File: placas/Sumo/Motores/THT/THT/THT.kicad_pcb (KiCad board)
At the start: 2 copper layers, 69.7 x 54.7 mm, 3 parts, among them J1 Control Motores, J2 Conn_01x02_Male

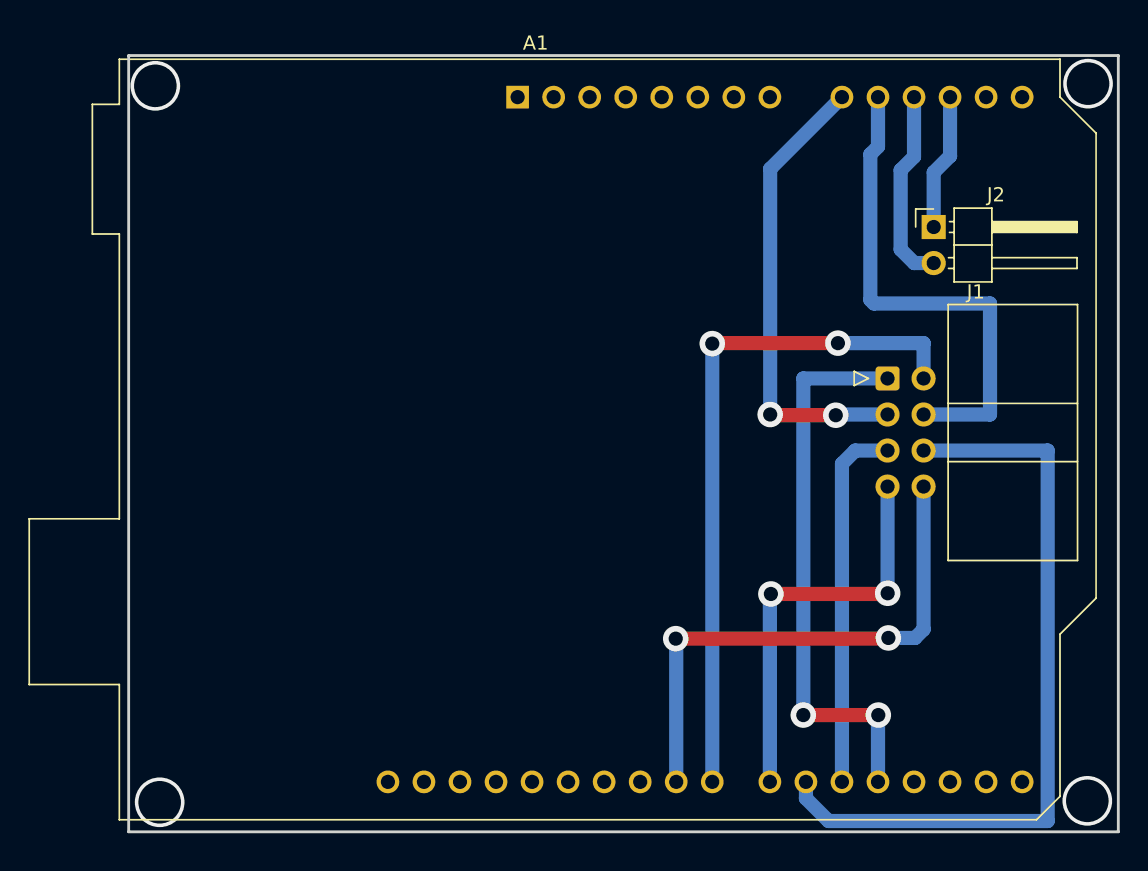
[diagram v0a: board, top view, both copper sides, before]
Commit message: CAMBIOS
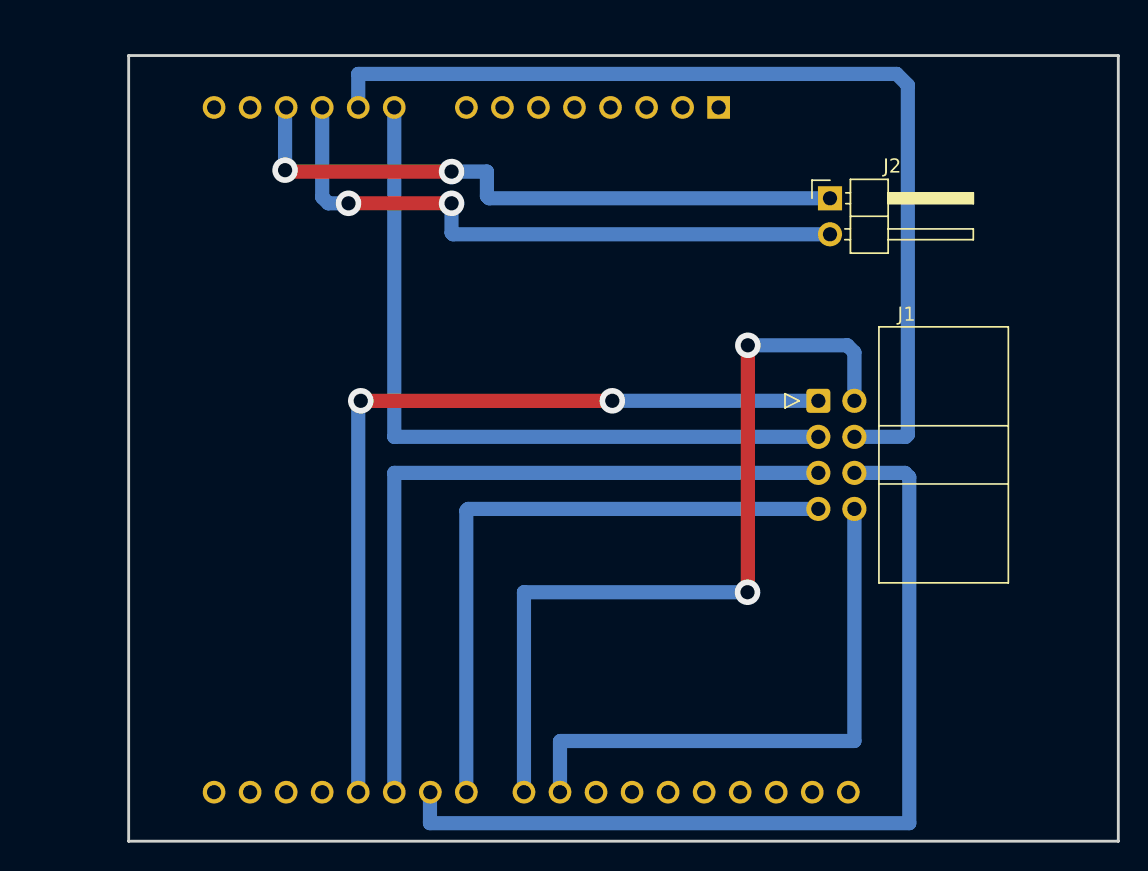
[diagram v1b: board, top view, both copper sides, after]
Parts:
- A1: moved to B.Cu
- moved A1 14.2 mm to (62.5, 20.2), turned to 180 degrees
- moved J2 7.58 mm to (70.4, 26.6)
- moved J1 5.12 mm to (69.5, 40.8)
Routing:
- net /C2: track 9.63 -> 44.7 mm, vias 0 -> 2
- net /EN2: track 35.6 -> 69.9 mm
- net /C1: track 13.9 -> 44.4 mm, vias 0 -> 2
- net /PWM1: track 26.0 -> 52.4 mm
- net /EN1: track 32.8 -> 53.1 mm, vias 2 -> 0
- net /INB1: track 39.7 -> 59.9 mm
- net /INA1: track 29.0 -> 44.7 mm, vias 2 -> 0
- net /PWM2: track 53.7 -> 64.4 mm
- net /INA2: track 48.3 -> 58.4 mm
- net /INB2: track 37.9 -> 40.7 mm, vias 2 -> 0
- net (no net): vias 4 -> 0
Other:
- board size 69.7 x 54.7 mm -> 69.7 x 55.4 mm
